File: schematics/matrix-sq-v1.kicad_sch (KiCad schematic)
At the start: 153 parts, among them J1 trg in 2, J2 trg in 1, J3 CV1, J4 CV2, J5 CV3, J6 Power, J7 Conn_01x02_Female, Q1 Q_NPN_BCE, Q2 Q_NPN_BCE, SW1 SW_Push, SW2 SW_Push, SW3 SW_Push, SW4 SW_Push, U1 TL084, X1 SW_Push, X2 SW_Push, X3 SW_Push, X4 SW_Push, X5 SW_Push, X6 SW_Push, Y1 SW_Push, Y2 SW_Push, Y3 SW_Push, Y4 SW_Push, Y5 SW_Push, Y6 SW_Push, Y7 Crystal

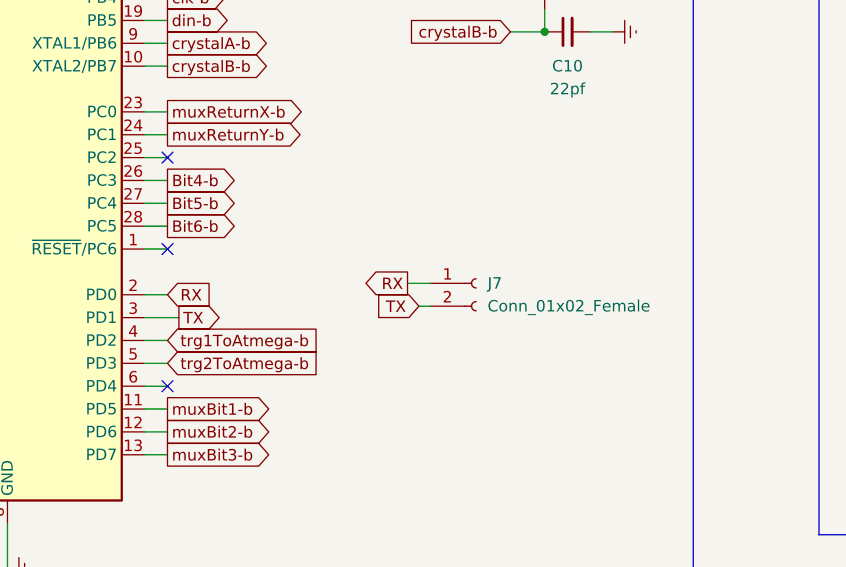
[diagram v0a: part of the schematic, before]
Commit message: refactor
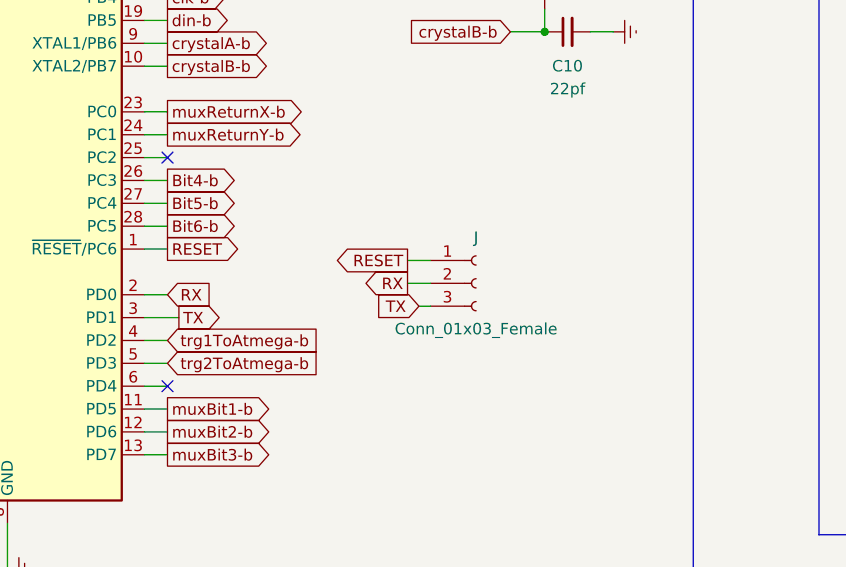
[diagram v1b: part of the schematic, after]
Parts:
- J: renamed from J7; value Conn_01x02_Female -> Conn_01x03_Female; footprint Connector_PinHeader_2.54mm:PinHeader_1x02_P2.54mm_Vertical -> Connector_PinHeader_2.54mm:PinHeader_1x03_P2.54mm_Vertical; symbol Connector:Conn_01x02_Female -> Connector:Conn_01x03_Female
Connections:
- net RX: now also J.2 (Pin_2); no longer J.1 (Pin_1)
- net TX: now also J.3 (Pin_3); no longer J.2 (Pin_2)
- net RESET: now reaches Atmega1.1 (~{RESET}/PC6)
- net RESET: now also J.1 (Pin_1)
- no-connect marks 9 -> 8
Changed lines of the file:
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@@
   )
   (no_connect (at 196.85 344.17))
-  (no_connect (at 425.45 92.71))
   (no_connect (at 196.85 341.63))
   (no_connect (at 196.85 361.95))
@@
     (stroke (width 0) (type default) (color 0 0 0 0))
   )
-  (wire (pts (xy 425.45 92.71) (xy 422.91 92.71))
-    (stroke (width 0) (type default) (color 0 0 0 0))
-  )
   (wire (pts (xy 248.92 260.35) (xy 255.27 260.35))
     (stroke (width 0) (type default) (color 0 0 0 0))
@@
     (stroke (width 0) (type default) (color 0 0 0 0))
   )
+  (wire (pts (xy 452.12 93.98) (xy 454.66 93.98))
+    (stroke (width 0) (type default) (color 0 0 0 0))
+  )
   (polyline (pts (xy 163.83 236.22) (xy 163.83 375.92))
     (stroke (width 0) (type default) (color 0 0 0 0))
@@
     (stroke (width 0) (type default) (color 0 0 0 0))
   )
+  (wire (pts (xy 425.45 92.71) (xy 422.91 92.71))
+    (stroke (width 0) (type default) (color 0 0 0 0))
+  )
   (wire (pts (xy 391.16 189.23) (xy 393.7 189.23))
     (stroke (width 0) (type default) (color 0 0 0 0))
@@
     )
   )
+  (global_label "RESET" (shape output) (at 452.12 93.98 180) (fields_autoplaced)
+    (effects (font (size 1.27 1.27)) (justify right))
+    (property "Referenzen zwischen Schaltplänen" "${INTERSHEET_REFS}" (id 0) (at 443.9617 93.9006 0)
+      (effects (font (size 1.27 1.27)) (justify right) hide)
+    )
+  )
   (global_label "Row3" (shape input) (at 73.66 298.45 180) (fields_autoplaced)
     (effects (font (size 1.27 1.27)) (justify right))
@@
     )
   )
+  (global_label "RESET" (shape output) (at 425.45 92.71 0) (fields_autoplaced)
+    (effects (font (size 1.27 1.27)) (justify left))
+    (property "Referenzen zwischen Schaltplänen" "${INTERSHEET_REFS}" (id 0) (at 433.6083 92.6306 0)
+      (effects (font (size 1.27 1.27)) (justify left) hide)
+    )
+  )
   (global_label "trg2ToAtmega-b" (shape input) (at 425.45 105.41 0) (fields_autoplaced)
     (effects (font (size 1.27 1.27)) (justify left))
@@
     (pin "2")
   )
-  (symbol (lib_id "Connector:Conn_01x02_Female") (at 459.74 96.52 0) (unit 1)
+  (symbol (lib_id "Connector:Conn_01x03_Female") (at 459.74 96.52 0) (unit 1)
     (in_bom yes) (on_board yes) (fields_autoplaced)
-    (property "Reference" "J7" (id 0) (at 461.01 96.5199 0)
-      (effects (font (size 1.27 1.27)) (justify left))
-    )
-    (property "Value" "Conn_01x02_Female" (id 1) (at 461.01 99.0599 0)
-      (effects (font (size 1.27 1.27)) (justify left))
-    )
-    (property "Footprint" "Connector_PinHeader_2.54mm:PinHeader_1x02_P2.54mm_Vertical" (id 2) (at 459.74 96.52 0)
+    (property "Reference" "J7" (id 0) (at 459.74 91.44 0))
+    (property "Value" "Conn_01x03_Female" (id 1) (at 459.74 101.6 0))
+    (property "Footprint" "Connector_PinHeader_2.54mm:PinHeader_1x03_P2.54mm_Vertical" (id 2) (at 459.74 96.52 0)
       (effects (font (size 1.27 1.27)) hide)
     )
@@
       (effects (font (size 1.27 1.27)) hide)
     )
-    (property "Reference" "J?" (id 5) (at 459.74 96.52 0)
-      (effects (font (size 1.27 1.27)) hide)
-    )
-    (property "Value" "Conn_01x02_Female" (id 6) (at 459.74 96.52 0)
-      (effects (font (size 1.27 1.27)) hide)
-    )
+    (property "Reference" "J" (id 5) (at 459.74 91.44 0))
+    (property "Value" "Conn_01x03_Female" (id 6) (at 459.74 101.6 0))
     (pin "1")
     (pin "2")
+    (pin "3")
   )
   (symbol (lib_id "power:Earth") (at 139.7 34.29 0) (unit 1)
@@
     )
     (path "/8466e8ee-285b-4d22-85cb-418892ae7734"
-      (reference "J7") (unit 1) (value "Conn_01x02_Female") (footprint "Connector_PinHeader_2.54mm:PinHeader_1x02_P2.54mm_Vertical")
+      (reference "J7") (unit 1) (value "Conn_01x03_Female") (footprint "Connector_PinHeader_2.54mm:PinHeader_1x03_P2.54mm_Vertical")
     )
     (path "/5c9d9677-b457-410a-bc69-748e427b7183"
